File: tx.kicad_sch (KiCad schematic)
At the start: 44 parts, among them J5 SWH, J7 SMA, T2 RF_BALUN, U12 MAX2831, U13 TXIF_BALUN, U16 DPDT

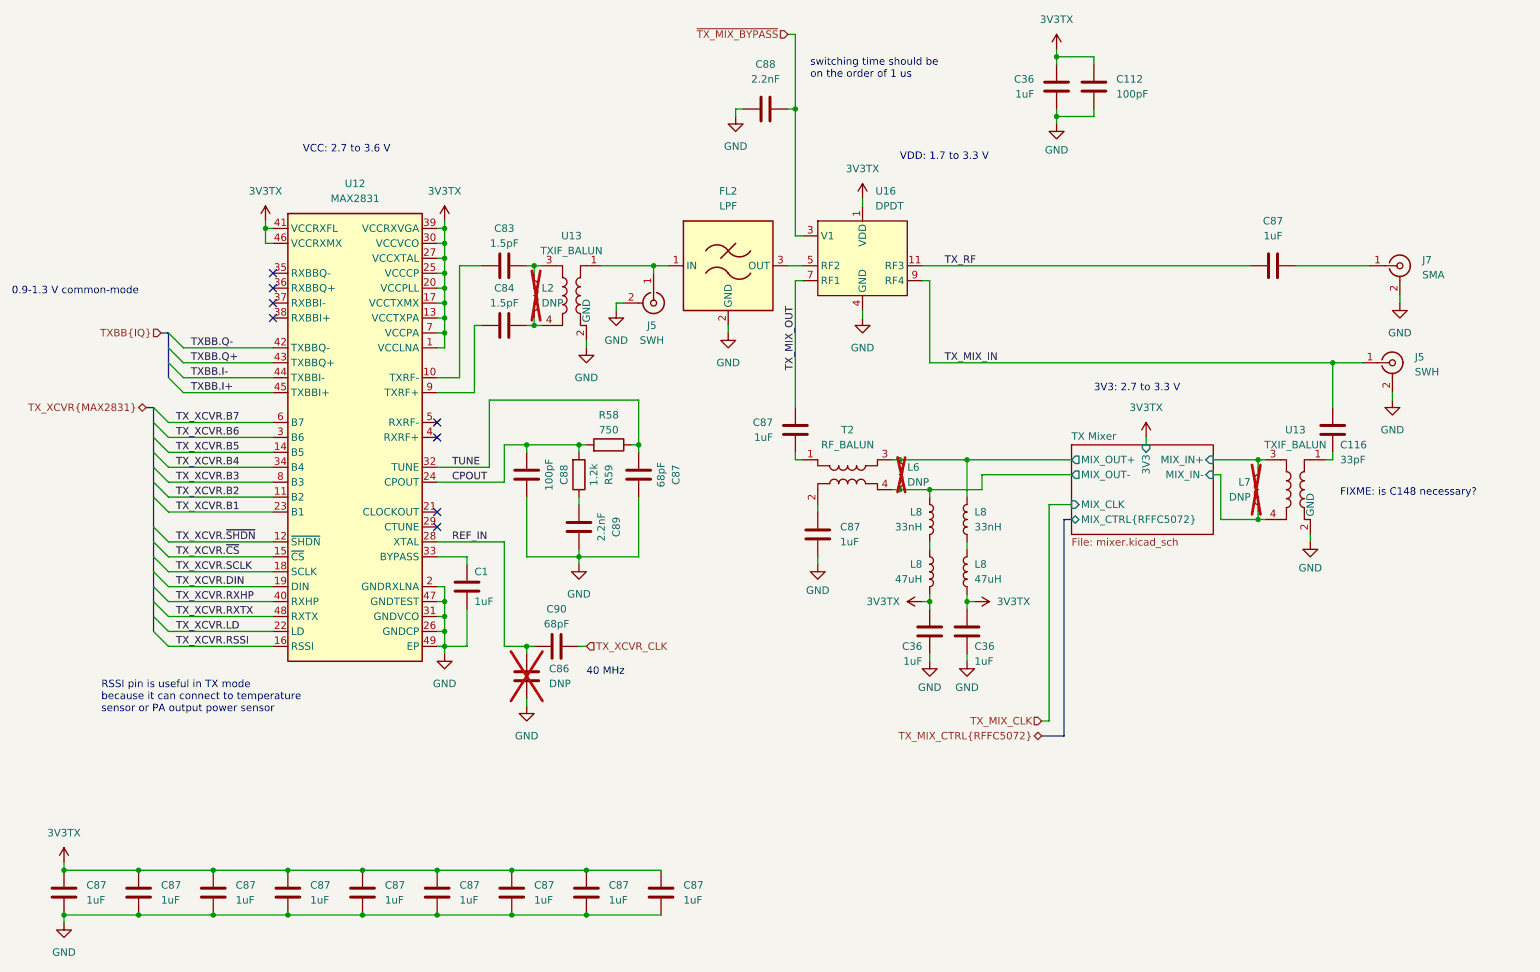
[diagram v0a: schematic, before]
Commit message: add SWH connector symbols
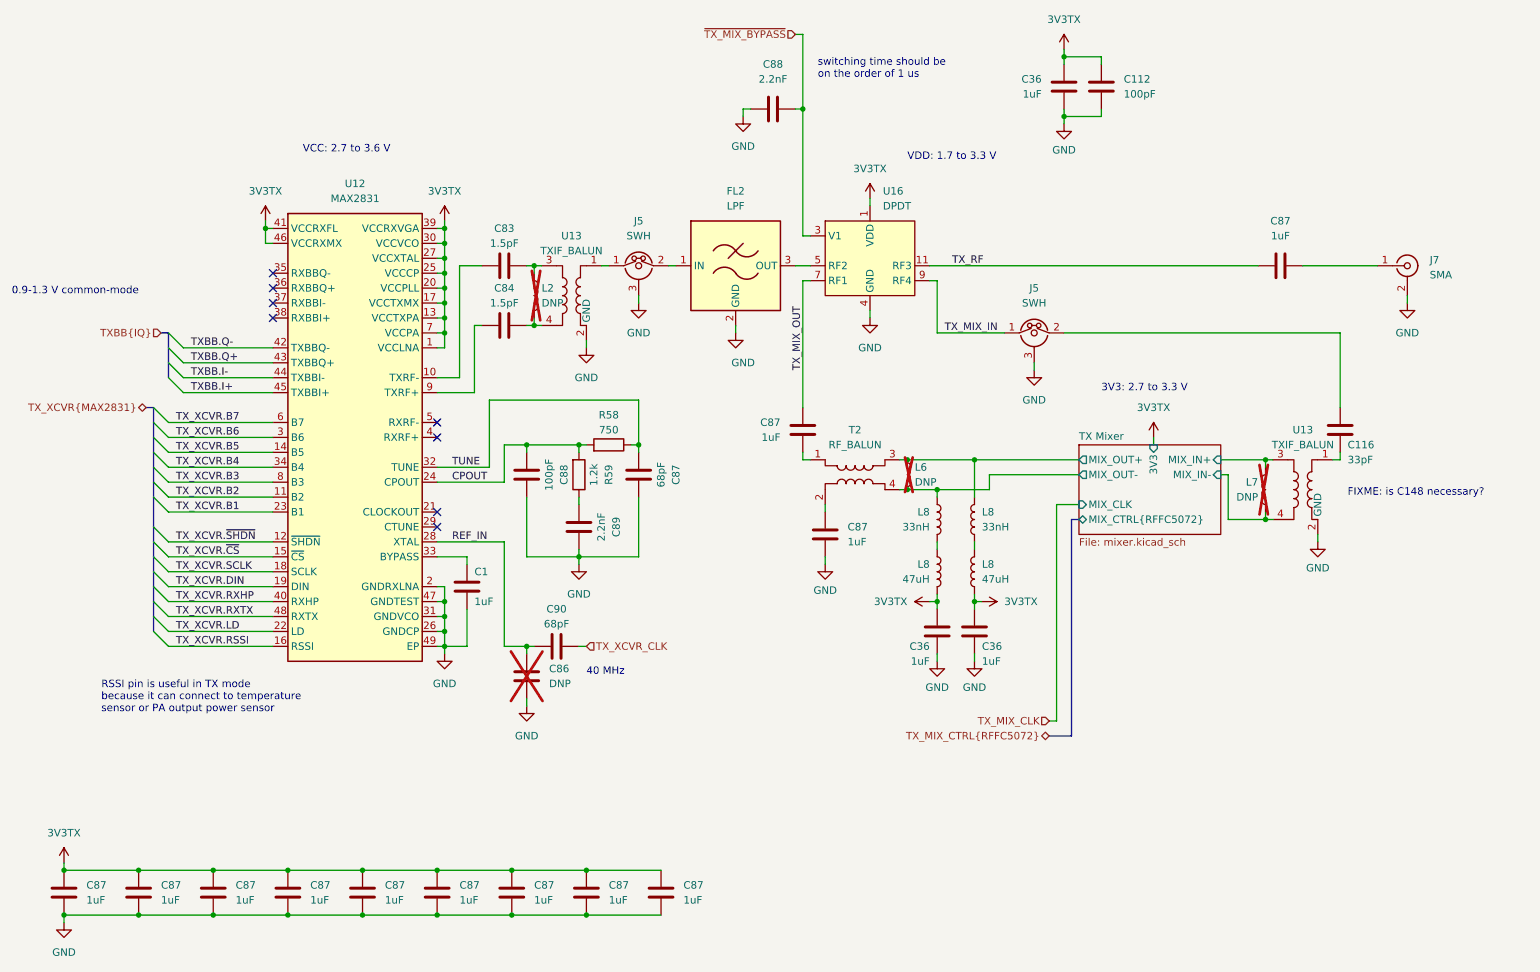
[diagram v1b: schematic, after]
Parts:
- removed J5 (x2): SWH, symbol Connector:Conn_Coaxial
- added J5 (x2): SWH, symbol radio:Conn_Coaxial_MM8930-2620
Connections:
- net GND: now also J5.3 (Ext), J5.3 (Ext)
- net TX_MIX_IN: now also J5.1 (C); no longer C116.1
- net at U13.1: now also J5.1 (C); no longer FL2.1 (IN)
- new net: C116.1, J5.2 (R)
- new net: FL2.1 (IN), J5.2 (R)
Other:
- moved on the sheet: C112, C116, C36, C87, C88, FL2, J7, L6, L7, L8, T2, U13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
